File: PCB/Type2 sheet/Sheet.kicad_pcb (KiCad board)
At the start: 2 copper layers, 111.3 x 96.9 mm, 88 parts, among them P1 C_0201_0603Metric_Pad0.64x0.4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, P2 C_0201_0603Metric_Pad0.64x0.4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, P3 C_0201_0603Metric_Pad0.64x0.4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, P4 C_0201_0603Metric_Pad0.64x0.4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, P5 C_0201_0603Metric_Pad0.64x0.4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, U1 MCP9700Ax-ELT, U10 ADS7830, U11 ADS7830, U12 MPU-6050, U2 MCP2562-E-MF, U3 ATtiny1616-M, U4 AP2112K-3.3, U5 CD74HC4067SM, U6 MCP2515-xST, U7 DRV5055A1xDBZxQ1, U8 DRV5055A1xDBZxQ1, U9 ADS7830

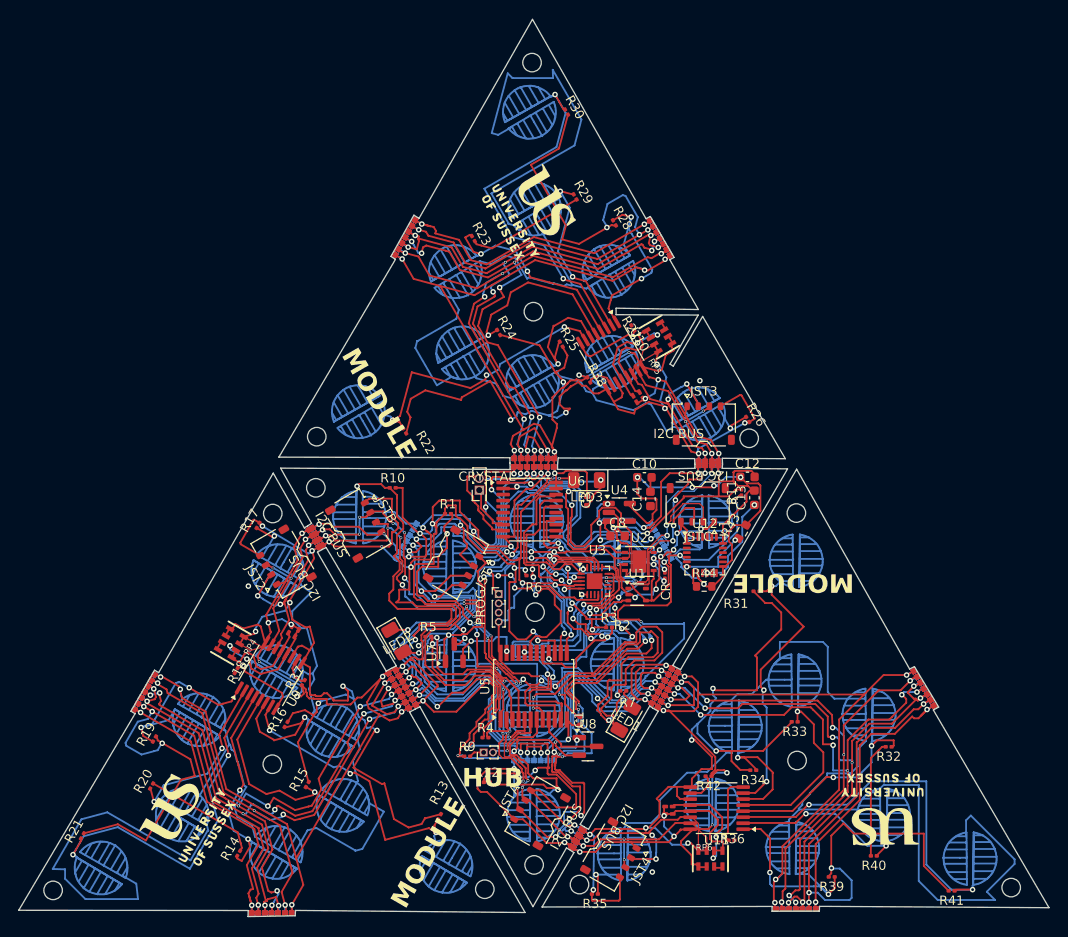
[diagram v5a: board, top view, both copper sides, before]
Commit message: fixes for manufacturing
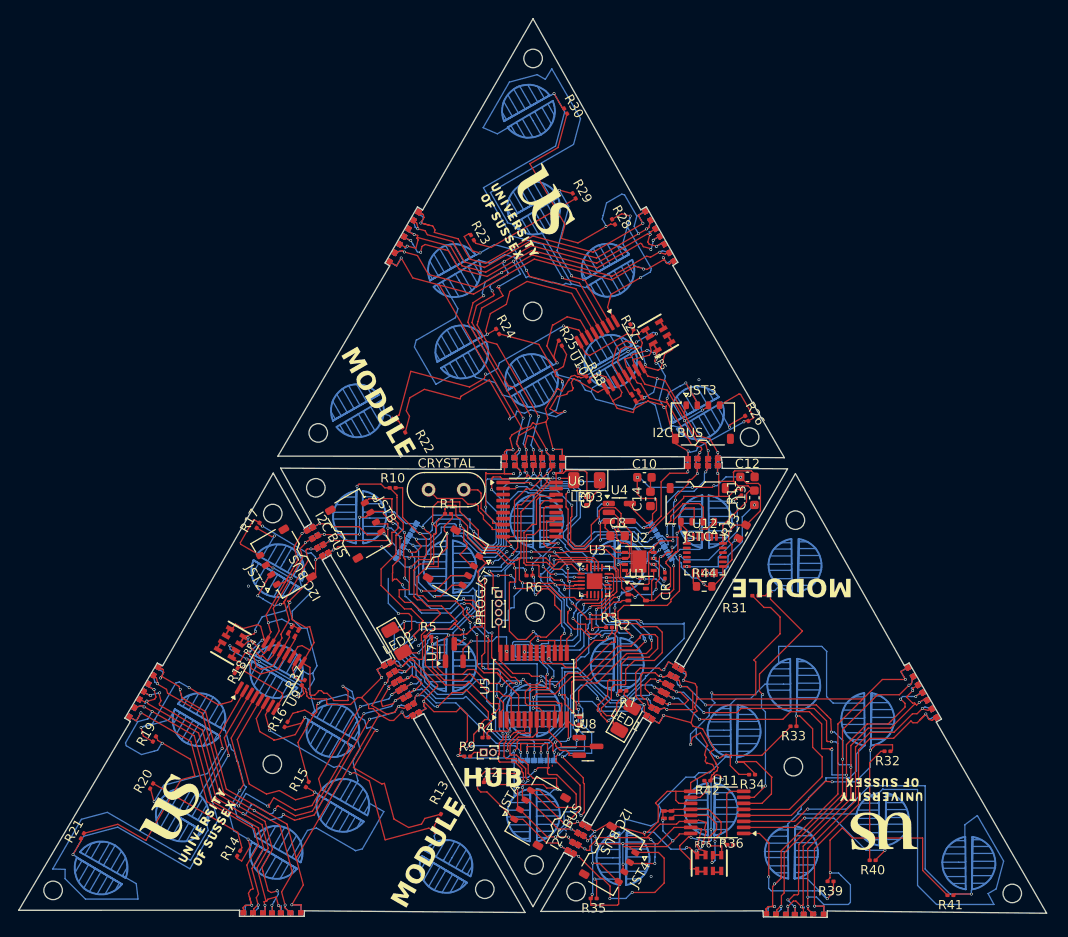
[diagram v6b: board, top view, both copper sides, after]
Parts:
- removed the CRYSTAL at (200.2, 104.8)
- added CRYSTAL: Crystal_HC52-6mm_Vertical, Crystal:Crystal_HC52-6mm_Vertical, F.Cu at (194.7, 104.8)
- R42: value 4.7k -> R
- moved JST4 0.50 mm to (214.5, 144.6)
- moved P5 0.50 mm to (220.5, 140.3)
- moved R32 0.50 mm to (244.2, 133.0)
- moved P4 0.50 mm to (220.5, 139.5)
- moved R33 0.50 mm to (234.1, 130.3)
- moved R40 0.50 mm to (242.6, 144.8)
- moved R34 0.50 mm to (229.6, 135.6)
- moved R41 0.50 mm to (251.0, 148.6)
- moved R35 0.50 mm to (212.5, 148.9)
- moved R39 0.50 mm to (238.1, 147.1)
- moved RP6 0.50 mm to (225.0, 145.1)
- moved R36 0.50 mm to (227.3, 143.1)
- moved R42 0.50 mm to (224.8, 136.2)
- moved G***2 0.50 mm to (243.7, 139.8)
- moved R31 0.50 mm to (230.0, 116.2)
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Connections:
- R22 pad 2: Net-(U10-CH1) -> Net-(U9-CH0)
- R23 pad 2: Net-(U10-CH2) -> Net-(U9-CH1)
- R24 pad 2: Net-(U10-CH3) -> Net-(U9-CH2)
- R25 pad 2: Net-(U10-CH4) -> Net-(U9-CH3)
- R26 pad 2: Net-(U10-CH5) -> Net-(U9-CH4)
- R27 pad 2: Net-(U10-CH6) -> Net-(U9-CH5)
- R28 pad 2: Net-(U10-CH7) -> Net-(U9-CH6)
- R29 pad 1: Net-(MK1--) -> unconnected-(R20-Pad1)
- R29 pad 2: Net-(U11-CH0) -> Net-(U9-CH7)
- R30 pad 2: Net-(U11-CH1) -> Net-(U10-CH0)
- R31 pad 2: Net-(U11-CH2) -> Net-(U9-CH0)
- R32 pad 2: Net-(U11-CH3) -> Net-(U9-CH1)
- R33 pad 2: Net-(U11-CH4) -> Net-(U9-CH2)
- R34 pad 2: Net-(U11-CH5) -> Net-(U9-CH3)
- R35 pad 2: Net-(U11-CH6) -> Net-(U9-CH4)
- R36 pad 2: Net-(U11-CH7) -> Net-(U9-CH5)
- R38 pad 2: Net-(U10-REFin/REFout) -> Net-(U9-REFin/REFout)
- R39 pad 1: Net-(U1-V_{DD}) -> Net-(MK1--)
- R39 pad 2: Net-(U11-REFin/REFout) -> Net-(U9-CH6)
- R40 pad 1: +3V3 -> unconnected-(R20-Pad1)
- R40 pad 2: Net-(D4-A) -> Net-(U9-CH7)
- R41 pad 1: +3V3 -> Net-(MK1--)
- R41 pad 2: /SCL -> Net-(U10-CH0)
- R42 pad 1: +3V3 -> Net-(U1-V_{DD})
- R42 pad 2: /SDA -> Net-(U9-REFin/REFout)
- U10 pad 1: Net-(U10-CH0) -> Net-(U9-CH0)
- U10 pad 10: Net-(U10-REFin/REFout) -> Net-(U9-REFin/REFout)
- U10 pad 12: unconnected-(U10-A0-Pad12) -> unconnected-(U9-A0-Pad12)
- U10 pad 13: unconnected-(U10-A1-Pad13) -> unconnected-(U9-A1-Pad13)
- U10 pad 2: Net-(U10-CH1) -> Net-(U9-CH1)
- U10 pad 3: Net-(U10-CH2) -> Net-(U9-CH2)
- U10 pad 4: Net-(U10-CH3) -> Net-(U9-CH3)
- U10 pad 5: Net-(U10-CH4) -> Net-(U9-CH4)
- U10 pad 6: Net-(U10-CH5) -> Net-(U9-CH5)
- U10 pad 7: Net-(U10-CH6) -> Net-(U9-CH6)
- U10 pad 8: Net-(U10-CH7) -> Net-(U9-CH7)
- U11 pad 1: Net-(U11-CH0) -> Net-(U9-CH0)
- U11 pad 10: Net-(U11-REFin/REFout) -> Net-(U9-REFin/REFout)
- U11 pad 12: unconnected-(U11-A0-Pad12) -> unconnected-(U9-A0-Pad12)
- U11 pad 13: unconnected-(U11-A1-Pad13) -> unconnected-(U9-A1-Pad13)
- U11 pad 2: Net-(U11-CH1) -> Net-(U9-CH1)
- U11 pad 3: Net-(U11-CH2) -> Net-(U9-CH2)
- U11 pad 4: Net-(U11-CH3) -> Net-(U9-CH3)
- U11 pad 5: Net-(U11-CH4) -> Net-(U9-CH4)
- U11 pad 6: Net-(U11-CH5) -> Net-(U9-CH5)
- U11 pad 7: Net-(U11-CH6) -> Net-(U9-CH6)
- U11 pad 8: Net-(U11-CH7) -> Net-(U9-CH7)
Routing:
- net (no net): track 2907.1 -> 1211.9 mm, vias 183 -> 74
- net Net-(MK1--): track 530.0 -> 1216.2 mm, vias 49 -> 64
- net Net-(U1-V_{DD}): track 499.0 -> 1055.6 mm, vias 58 -> 120
- net Net-(U2-CANL): track 0.00 -> 326.2 mm, vias 0 -> 32
- net Net-(U9-CH2): track 39.1 -> 117.3 mm, vias 2 -> 6
- net Net-(U11-CH2): track 52.8 -> 0.00 mm, vias 2 -> 0
- net Net-(U9-CH3): track 21.7 -> 65.1 mm, vias 2 -> 6
- net Net-(U9-CH4): track 38.3 -> 77.7 mm, vias 1 -> 3
- net Net-(U9-CH1): track 51.0 -> 90.0 mm, vias 2 -> 6
- net Net-(U11-CH1): track 33.2 -> 0.00 mm, vias 2 -> 0
- net Net-(U9-CH0): track 136.8 -> 166.8 mm, vias 7 -> 9
- net Net-(U2-RXD): track 0.00 -> 29.1 mm, vias 0 -> 2
- net unconnected-(U9-A0-Pad12): track 12.0 -> 36.0 mm, vias 2 -> 6
- net Net-(U11-CH7): track 22.7 -> 0.00 mm, vias 1 -> 0
- net unconnected-(U9-A1-Pad13): track 10.4 -> 31.1 mm
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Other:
- board size 111.3 x 96.9 mm -> 111 x 97.1 mm
